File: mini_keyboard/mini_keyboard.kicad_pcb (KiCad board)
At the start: 2 copper layers, 4 parts, among them U1 MX1A-11NN, U2 MX1A-11NN, U3 MX1A-11NN, U4 MX1A-11NN

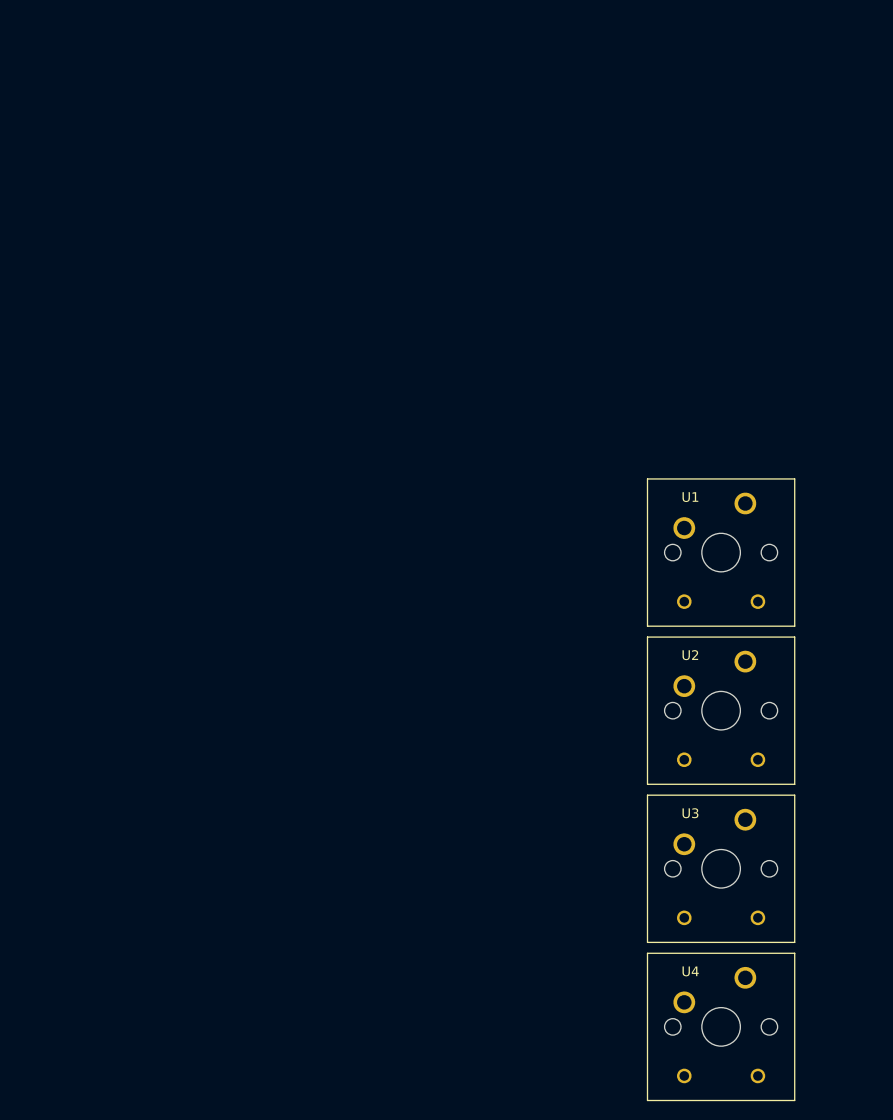
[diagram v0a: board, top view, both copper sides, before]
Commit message: adding more keys and looking at spacing
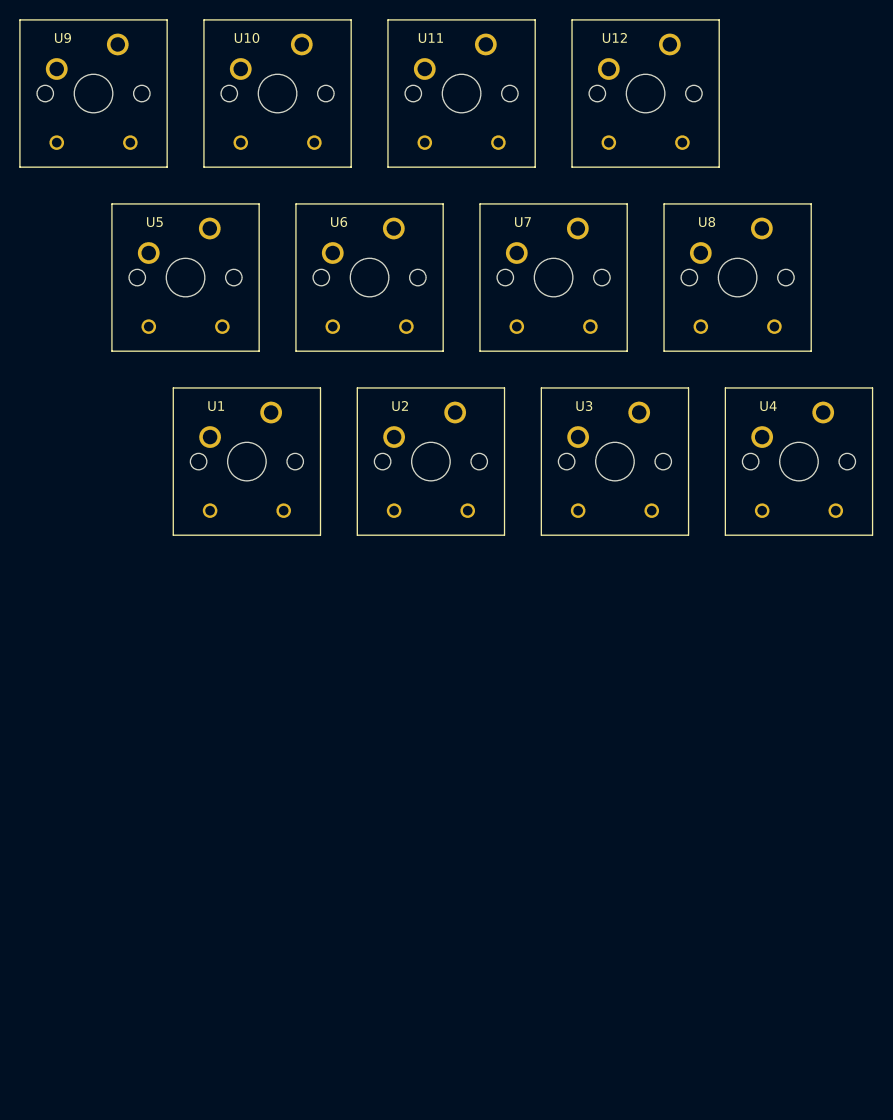
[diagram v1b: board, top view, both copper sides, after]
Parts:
- added U10: MX1A-11NN, pedrolib:CHERRY_MX1A-11NN_SWITCH, F.Cu at (54.0, 25.4)
- added U11: MX1A-11NN, pedrolib:CHERRY_MX1A-11NN_SWITCH, F.Cu at (73.0, 25.4)
- added U12: MX1A-11NN, pedrolib:CHERRY_MX1A-11NN_SWITCH, F.Cu at (92.1, 25.4)
- added U5: MX1A-11NN, pedrolib:CHERRY_MX1A-11NN_SWITCH, F.Cu at (44.5, 44.5)
- added U6: MX1A-11NN, pedrolib:CHERRY_MX1A-11NN_SWITCH, F.Cu at (63.5, 44.5)
- added U7: MX1A-11NN, pedrolib:CHERRY_MX1A-11NN_SWITCH, F.Cu at (82.5, 44.5)
- added U8: MX1A-11NN, pedrolib:CHERRY_MX1A-11NN_SWITCH, F.Cu at (101.6, 44.5)
- added U9: MX1A-11NN, pedrolib:CHERRY_MX1A-11NN_SWITCH, F.Cu at (34.9, 25.4)
- moved U4 59.1 mm to (108.0, 63.5)
- moved U1 50.0 mm to (50.8, 63.5)
- moved U3 43.6 mm to (88.9, 63.5)
- moved U2 39.6 mm to (69.8, 63.5)
